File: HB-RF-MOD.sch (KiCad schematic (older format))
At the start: 25 parts, among them J1 RPi Header, J2 RGB, Q1 BC847, SW1 Button, U1 TRX2-TIF, U2 RX8130-CE, U3 3V3LDO

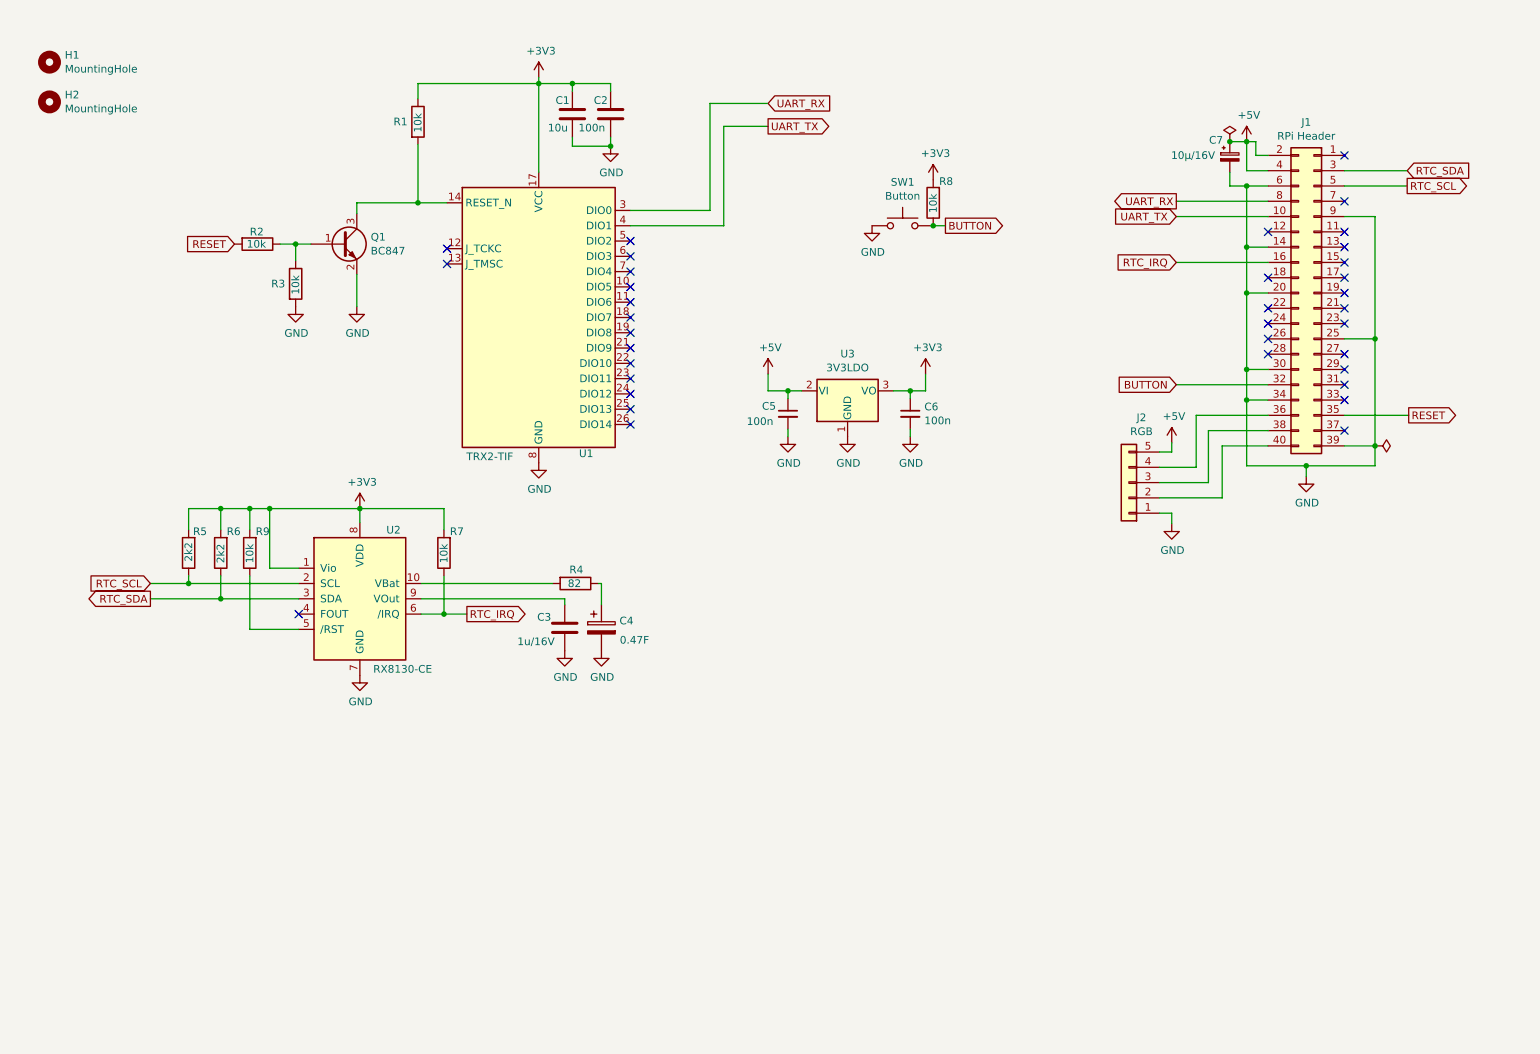
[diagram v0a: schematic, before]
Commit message: update
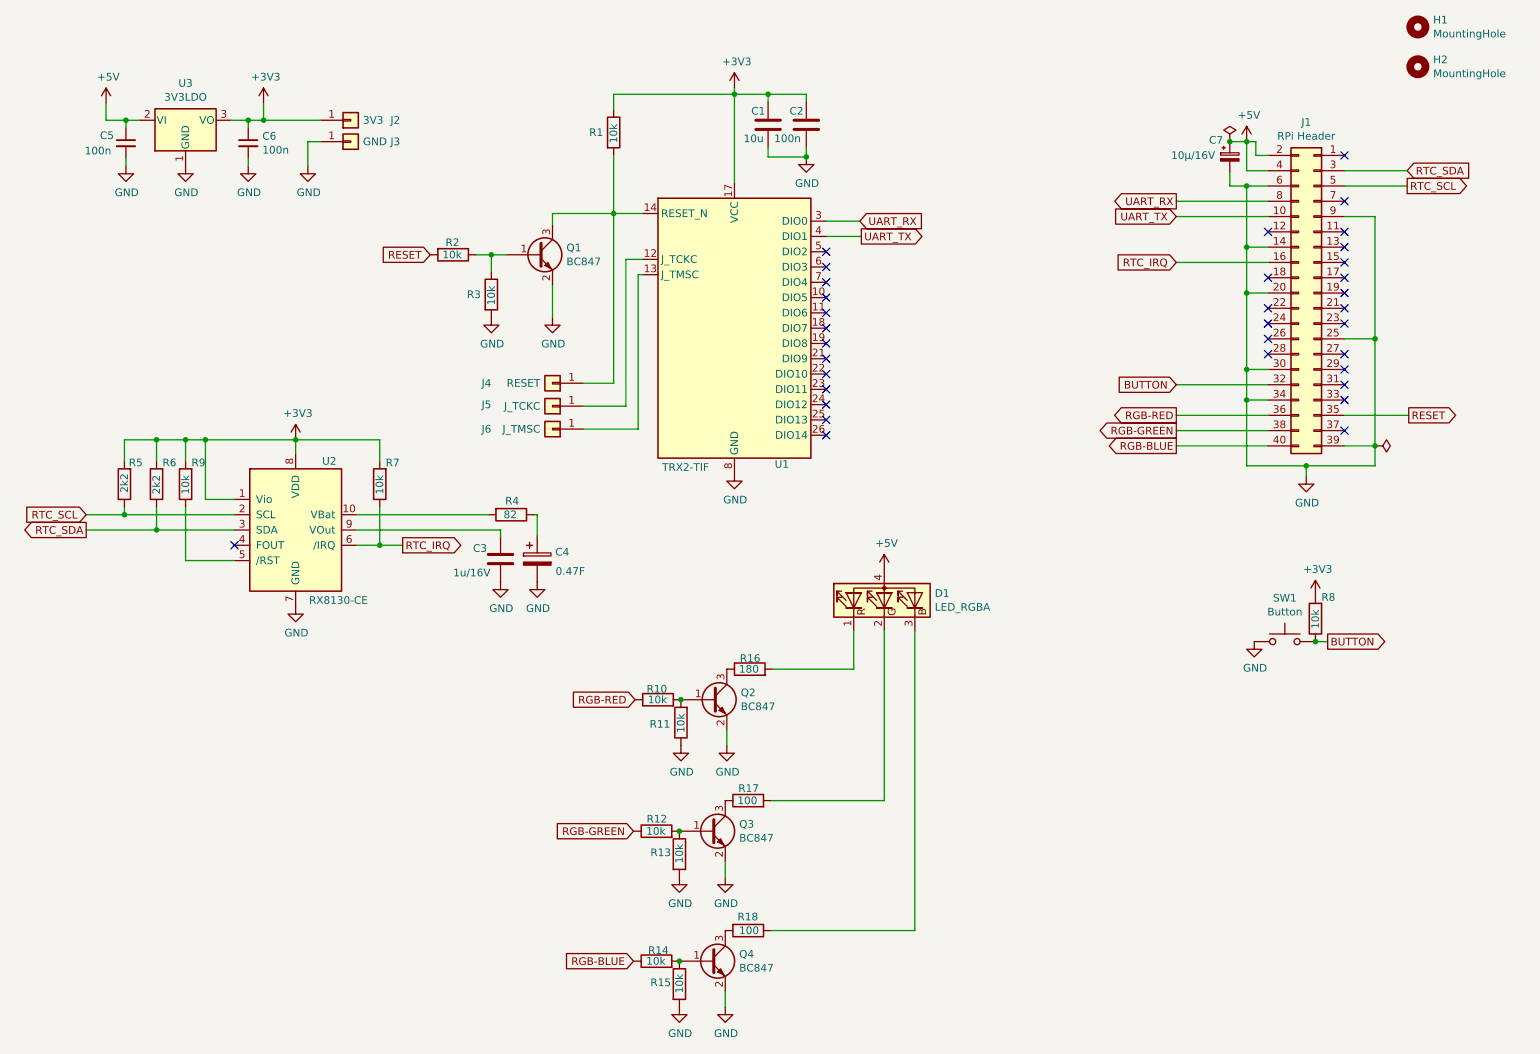
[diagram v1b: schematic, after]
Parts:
- removed J2: RGB, Connector_PinHeader_2.00mm:PinHeader_1x05_P2.00mm_Vertical, symbol Connector_Generic:Conn_01x05
- added D1: LED_RGBA, LED_THT:LED_D5.0mm-4_RGB_Wide_Pins, symbol Device:LED_RGBA
- added J2: 3V3, TestPoint:TestPoint_Pad_D1.5mm, symbol Connector_Generic:Conn_01x01
- added J3: GND, TestPoint:TestPoint_Pad_D1.5mm, symbol Connector_Generic:Conn_01x01
- added J4: RESET, TestPoint:TestPoint_Pad_D1.5mm, symbol Connector_Generic:Conn_01x01
- added J5: J_TCKC, TestPoint:TestPoint_Pad_D1.5mm, symbol Connector_Generic:Conn_01x01
- added J6: J_TMSC, TestPoint:TestPoint_Pad_D1.5mm, symbol Connector_Generic:Conn_01x01
- added Q2, Q3, Q4: BC847, Package_TO_SOT_SMD:SOT-23, symbol Transistor_BJT:BC847
- added R10, R11, R12, R13, R14, R15: 10k, Resistor_SMD:R_0805_2012Metric_Pad1.15x1.40mm_HandSolder, symbol Device:R
- added R16: 180, Resistor_SMD:R_0805_2012Metric_Pad1.15x1.40mm_HandSolder, symbol Device:R
- added R17, R18: 100, Resistor_SMD:R_0805_2012Metric_Pad1.15x1.40mm_HandSolder, symbol Device:R
- C4: footprint Capacitor_THT:CP_Radial_D22.0mm_P10.00mm_SnapIn -> additional:CP_Radial_D20.0mm_P5.00mm
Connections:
- net +3V3: now also J2.1 (Pin_1)
- net +5V: now also D1.4 (A)
- net GND: now also J3.1 (Pin_1), Q2.2 (E), Q3.2 (E), Q4.2 (E), R11.1, R13.2, R15.2
- net at Q1.3 (C), R1.2, U1.14 (RESET_N): now also J4.1 (Pin_1)
- net at U1.12 (J_TCKC): now also J5.1 (Pin_1)
- net at U1.13 (J_TMSC): now also J6.1 (Pin_1)
- net RGB-RED: now reaches J1.36 (Pin_36)
- net RGB-RED: now also R10.1
- net RGB-GREEN: now reaches J1.38 (Pin_38)
- net RGB-GREEN: now also R12.1
- net RGB-BLUE: now reaches J1.40 (Pin_40)
- net RGB-BLUE: now also R14.1
- new net: Q3.1 (B), R12.2, R13.1
- new net: Q4.1 (B), R14.2, R15.1
- new net: Q2.1 (B), R10.2, R11.2
- new net: D1.3 (BK), R18.1
- new net: Q4.3 (C), R18.2
- new net: Q2.3 (C), R16.1
- new net: D1.1 (RK), R16.2
- new net: Q3.3 (C), R17.1
- new net: D1.2 (GK), R17.2
- no-connect marks 36 -> 34
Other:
- moved on the sheet: C1, C2, C3, C4, C5, C6, H1, H2, Q1, R1, R2, R3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
